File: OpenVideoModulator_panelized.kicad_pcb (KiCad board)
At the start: 2 copper layers, 99.2 x 91 mm, 182 parts, among them J1 CONN_6, J1 CONN_7, J1 Conn_01x08, J2 CONN_6, J2 CONN_7, J2 Conn_02x08_Counter_Clockwise, J3 Conn_01x08, J3 RCA, J4 Mini-DIN-4, J5 Conn_01x04_Male, J6 Barrel_Jack, P1 OSHW_LOGO, U1 AD724, Y1 4.433619M

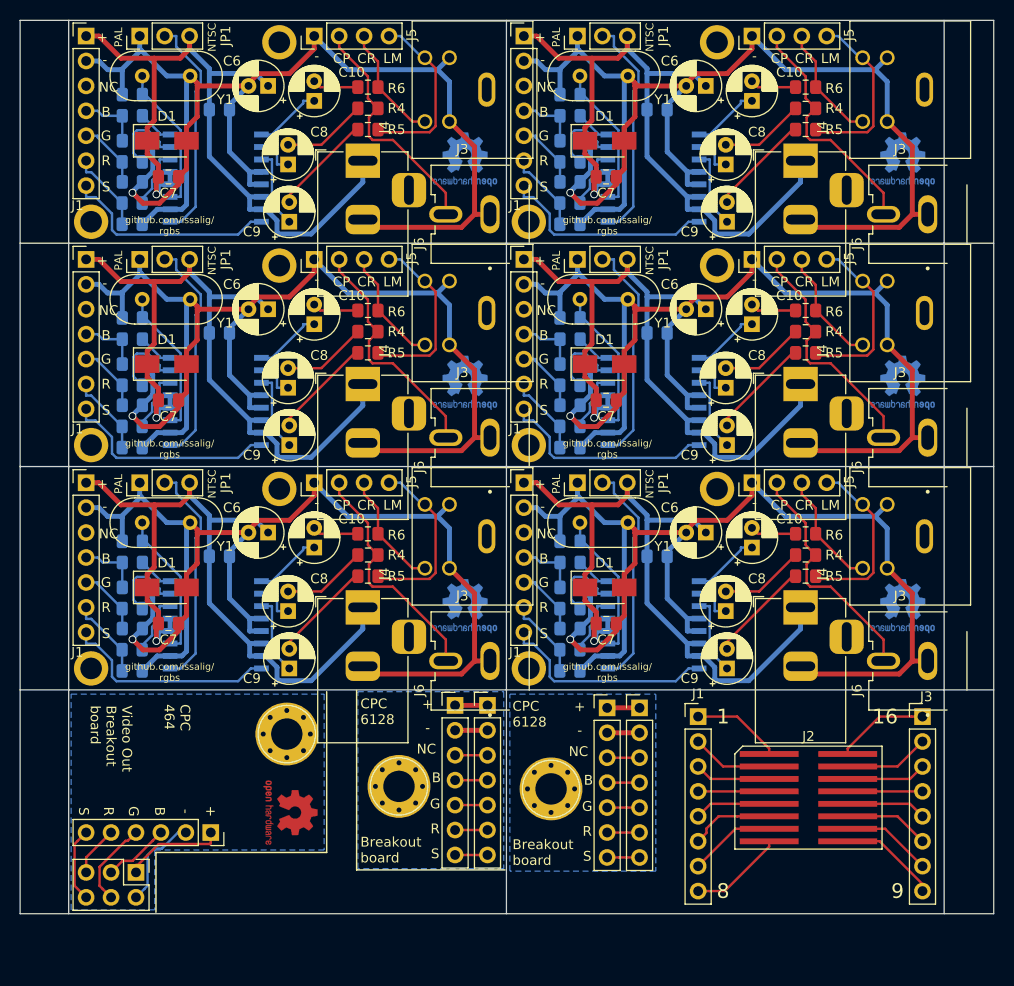
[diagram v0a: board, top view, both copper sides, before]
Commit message: rgbs
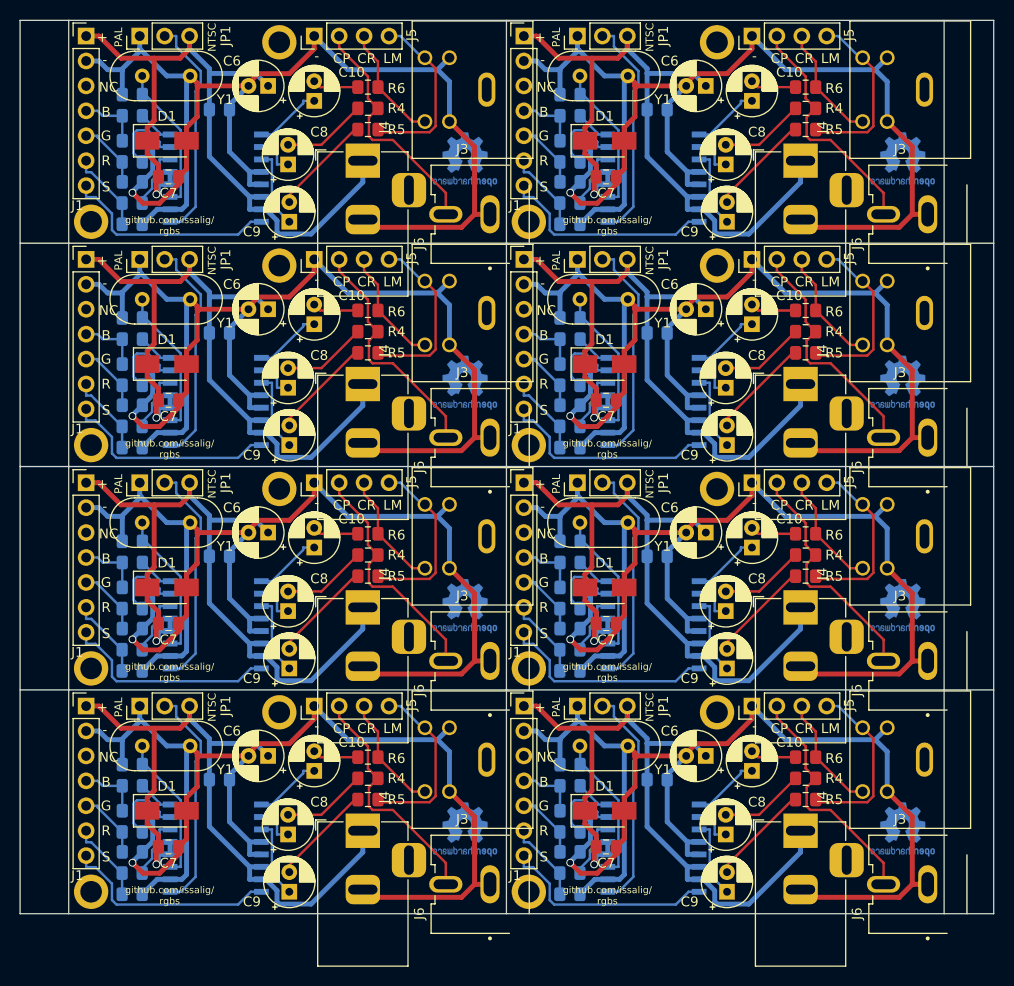
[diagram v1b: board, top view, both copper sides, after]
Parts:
- removed the H1 at (147.6, 127.8)
- removed the H1 at (136.1, 122.4)
- removed the H1 at (163.1, 128.0)
- removed the J1 at (172.1, 119.8)
- removed the J1 at (156.6, 119.5)
- removed the J1 at (120.8, 136.5)
- removed the J1 at (178.1, 120.7)
- removed J2 (x2): CONN_7, Connector_PinHeader_2.54mm:PinHeader_1x07_P2.54mm_Vertical
- removed J2: CONN_6, Connector_PinSocket_2.54mm:PinSocket_1x06_P2.54mm_Vertical
- removed J2: Conn_02x08_Counter_Clockwise, open:SOIC-16
- removed the J3 at (200.9, 120.7)
- removed the J6 at (143.9, 109.5)
- removed REF**: KiCad-Logo2_5mm_SilkScreen, Symbol:KiCad-Logo2_5mm_SilkScreen
- removed REF**: OSHW-Logo2_7.3x6mm_Copper, Symbol:OSHW-Logo2_7.3x6mm_Copper
- added C1: 10pF, Capacitor_SMD:C_0805_2012Metric_Pad1.15x1.40mm_HandSolder, B.Cu at (165.0, 125.5)
- added C1: 10pF, Capacitor_SMD:C_0805_2012Metric_Pad1.15x1.40mm_HandSolder, B.Cu at (120.4, 125.5)
- added C10: 220u, Capacitor_THT:CP_Radial_D5.0mm_P2.00mm, F.Cu at (183.5, 126.2)
- added C10: 220u, Capacitor_THT:CP_Radial_D5.0mm_P2.00mm, F.Cu at (138.9, 126.2)
- added C2: 100n, Capacitor_SMD:C_0805_2012Metric_Pad1.15x1.40mm_HandSolder, B.Cu at (165.0, 136.6)
- added C2: 100n, Capacitor_SMD:C_0805_2012Metric_Pad1.15x1.40mm_HandSolder, B.Cu at (120.4, 136.6)
- added C3: 100n, Capacitor_SMD:C_0805_2012Metric_Pad1.15x1.40mm_HandSolder, B.Cu at (165.0, 132.4)
- added C3: 100n, Capacitor_SMD:C_0805_2012Metric_Pad1.15x1.40mm_HandSolder, B.Cu at (120.4, 132.4)
- added C4: 100n, Capacitor_SMD:C_0805_2012Metric_Pad1.15x1.40mm_HandSolder, B.Cu at (165.0, 127.7)
- added C4: 100n, Capacitor_SMD:C_0805_2012Metric_Pad1.15x1.40mm_HandSolder, B.Cu at (120.4, 127.7)
- added C5: 100n, Capacitor_SMD:C_0805_2012Metric_Pad1.15x1.40mm_HandSolder, B.Cu at (173.9, 127.1)
- added C5: 100n, Capacitor_SMD:C_0805_2012Metric_Pad1.15x1.40mm_HandSolder, B.Cu at (129.3, 127.1)
- added C6: 100u, Capacitor_THT:CP_Radial_D5.0mm_P2.00mm, F.Cu at (178.8, 124.7)
- added C6: 100u, Capacitor_THT:CP_Radial_D5.0mm_P2.00mm, F.Cu at (134.2, 124.7)
- added C7: 100n, Capacitor_SMD:C_0805_2012Metric_Pad1.15x1.40mm_HandSolder, F.Cu at (168.7, 133.9)
- added C7: 100n, Capacitor_SMD:C_0805_2012Metric_Pad1.15x1.40mm_HandSolder, F.Cu at (124.1, 133.9)
- added C8: 220u, Capacitor_THT:CP_Radial_D5.0mm_P2.00mm, F.Cu at (180.9, 132.7)
- added C8: 220u, Capacitor_THT:CP_Radial_D5.0mm_P2.00mm, F.Cu at (136.3, 132.7)
- added C9: 220u, Capacitor_THT:CP_Radial_D5.0mm_P2.00mm, F.Cu at (181.0, 138.5)
- added C9: 220u, Capacitor_THT:CP_Radial_D5.0mm_P2.00mm, F.Cu at (136.4, 138.5)
- added D1: 1N4001, Diode_SMD:D_SMA, F.Cu at (168.5, 130.2)
- added D1: 1N4001, Diode_SMD:D_SMA, F.Cu at (123.9, 130.2)
- added H1: MountingHole, MountingHole:MountingHole_2.2mm_M2_ISO7380_Pad, F.Cu at (160.8, 138.5)
- added H1: MountingHole, MountingHole:MountingHole_2.2mm_M2_ISO7380_Pad, F.Cu at (116.2, 138.5)
- added H2: MountingHole, MountingHole:MountingHole_2.2mm_M2_ISO7380_Pad, F.Cu at (180.0, 120.2)
- added H2: MountingHole, MountingHole:MountingHole_2.2mm_M2_ISO7380_Pad, F.Cu at (135.4, 120.2)
- added J1: CONN_7, Connector_PinHeader_2.54mm:PinHeader_1x07_P2.54mm_Vertical, F.Cu at (160.3, 119.6)
- added J1: CONN_7, Connector_PinHeader_2.54mm:PinHeader_1x07_P2.54mm_Vertical, F.Cu at (115.7, 119.6)
- added J3: RCA, OpenVideoModulator:CUI_RCJ-044, F.Cu at (201.4, 137.7)
- added J3: RCA, OpenVideoModulator:CUI_RCJ-044, F.Cu at (156.8, 137.7)
- added J4: Mini-DIN-4, OpenVideoModulator:CUI_MD-40S_1234, F.Cu at (199.7, 125.0)
- added J4: Mini-DIN-4, OpenVideoModulator:CUI_MD-40S_1234, F.Cu at (155.1, 125.0)
- added J5: Conn_01x04_Male, Connector_PinHeader_2.54mm:PinHeader_1x04_P2.54mm_Vertical, F.Cu at (183.5, 119.6)
- added J5: Conn_01x04_Male, Connector_PinHeader_2.54mm:PinHeader_1x04_P2.54mm_Vertical, F.Cu at (138.9, 119.6)
- added J6: Barrel_Jack, Connector_BarrelJack:BarrelJack_Horizontal, F.Cu at (188.5, 132.3)
- added J6: Barrel_Jack, Connector_BarrelJack:BarrelJack_Horizontal, F.Cu at (143.9, 132.3)
- added J6: Barrel_Jack, Connector_BarrelJack:BarrelJack_Horizontal, F.Cu at (143.9, 109.5)
- added JP1: NTSC/~PAL, Connector_PinHeader_2.54mm:PinHeader_1x03_P2.54mm_Vertical, F.Cu at (165.8, 119.6)
- added JP1: NTSC/~PAL, Connector_PinHeader_2.54mm:PinHeader_1x03_P2.54mm_Vertical, F.Cu at (121.2, 119.6)
- added P1: OSHW_LOGO, Symbol:OSHW-Logo2_7.3x6mm_Copper, B.Cu at (198.9, 132.1)
- added P1: OSHW_LOGO, Symbol:OSHW-Logo2_7.3x6mm_Copper, B.Cu at (154.3, 132.1)
- added R1: 75, Resistor_SMD:R_0805_2012Metric_Pad1.15x1.40mm_HandSolder, B.Cu at (165.0, 138.8)
- added R1: 75, Resistor_SMD:R_0805_2012Metric_Pad1.15x1.40mm_HandSolder, B.Cu at (120.4, 138.8)
- added R2: 75, Resistor_SMD:R_0805_2012Metric_Pad1.15x1.40mm_HandSolder, B.Cu at (165.0, 134.4)
- added R2: 75, Resistor_SMD:R_0805_2012Metric_Pad1.15x1.40mm_HandSolder, B.Cu at (120.4, 134.4)
- added R3: 75, Resistor_SMD:R_0805_2012Metric_Pad1.15x1.40mm_HandSolder, B.Cu at (165.0, 130.2)
- added R3: 75, Resistor_SMD:R_0805_2012Metric_Pad1.15x1.40mm_HandSolder, B.Cu at (120.4, 130.2)
- added R4: 75, Resistor_SMD:R_0805_2012Metric_Pad1.15x1.40mm_HandSolder, F.Cu at (189.0, 126.9)
- added R4: 75, Resistor_SMD:R_0805_2012Metric_Pad1.15x1.40mm_HandSolder, F.Cu at (144.4, 126.9)
- added R5: 75, Resistor_SMD:R_0805_2012Metric_Pad1.15x1.40mm_HandSolder, F.Cu at (189.0, 129.1)
- added R5: 75, Resistor_SMD:R_0805_2012Metric_Pad1.15x1.40mm_HandSolder, F.Cu at (144.4, 129.1)
- added R6: 75, Resistor_SMD:R_0805_2012Metric_Pad1.15x1.40mm_HandSolder, F.Cu at (189.0, 124.8)
- added R6: 75, Resistor_SMD:R_0805_2012Metric_Pad1.15x1.40mm_HandSolder, F.Cu at (144.4, 124.8)
- added U1: AD724, Package_SO:SOIC-16W_7.5x10.3mm_P1.27mm, B.Cu at (173.5, 134.1)
- added U1: AD724, Package_SO:SOIC-16W_7.5x10.3mm_P1.27mm, B.Cu at (128.9, 134.1)
- added Y1: 4.433619M, Crystal:Crystal_HC49-4H_Vertical, F.Cu at (170.9, 123.6)
- added Y1: 4.433619M, Crystal:Crystal_HC49-4H_Vertical, F.Cu at (126.3, 123.6)
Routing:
- net GND: track 825.7 -> 1079.2 mm, vias 6 -> 8
- net VAA: track 462.2 -> 616.2 mm, vias 6 -> 8
- net COMP: track 147.8 -> 197.1 mm
- net Net-(JP1-Pad2): track 138.3 -> 184.4 mm
- net LUMA: track 109.5 -> 146.0 mm
- net /sync_in: track 146.2 -> 177.0 mm
- net Net-(C1-Pad1): track 91.1 -> 121.5 mm
- net CRMA: track 72.2 -> 96.2 mm
- net Net-(C9-Pad2): track 62.8 -> 83.7 mm
- net VCC: track 18.0 -> 0.00 mm
- net Net-(C8-Pad2): track 51.9 -> 69.2 mm
- net Net-(C9-Pad1): track 48.9 -> 65.3 mm
- net Net-(C3-Pad1): track 48.8 -> 65.1 mm
- net Net-(C10-Pad1): track 41.7 -> 55.6 mm
- net Net-(C2-Pad1): track 37.5 -> 50.0 mm
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- removed copper zone on B.Cu, net GND
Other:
- board text added: "OpenVideoModulator_panelized.kicad_pcb (2x4 panel) generated with: ./panelizer.py --panelx=100 --panely=100 --hrail=5 OpenVideoModulator.kicad_pcb"
- board text removed: "../OpenVideoModulator/OpenVideoModulator_panelized.kicad_pcb (2x4 panel) generated with: ./panelizer.py --panelx=100 --panely=100 --hrail=5 ../OpenVideoModulator/OpenVideoModulator.kicad_pcb"
- board text removed: "1"
- board text removed: "16"
- board text removed: "8"
- board text removed: "9"
- board text removed: "Breakout board"
- board text removed: "CPC 464"
- board text removed: "CPC 6128"
- board text removed: "Video Out Breakout board"
- board text removed: "github.com /issalig/ rgbs"
- board text removed: "github.com/ issalig/rgbs 3/2021"
